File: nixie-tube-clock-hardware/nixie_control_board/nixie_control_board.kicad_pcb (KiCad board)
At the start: 2 copper layers, 52.5 x 97 mm, 62 parts, among them J1 Conn_01x07, P1 CONN_01X02, P2 CONN_01X02, P3 AMS1117, P4 CONN_01X02, P6 CONN_01X02, P7 CONN_01X02, Q1 IRF644, SW4 SW_DIP_x01, U1 DS3231, U2 AT24C02, U3 MAX1771, U7 SSD1306-OLED, U8 MP2307

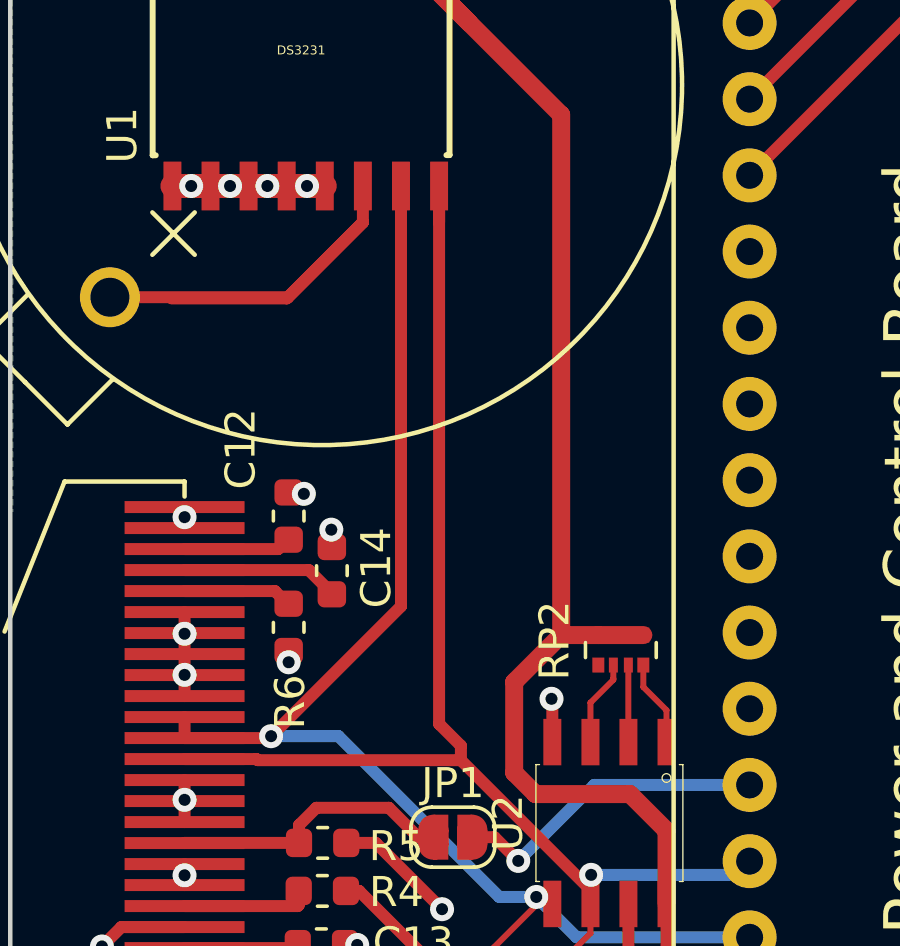
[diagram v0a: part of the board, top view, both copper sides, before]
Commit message: Some hardware changes
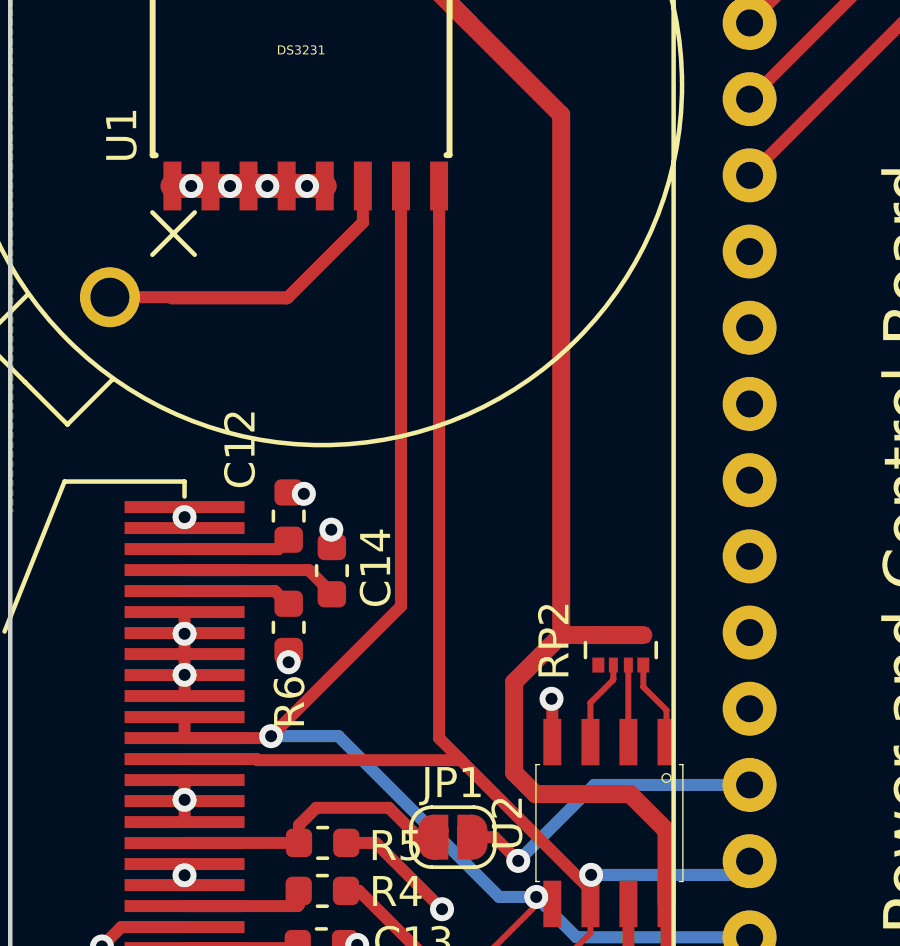
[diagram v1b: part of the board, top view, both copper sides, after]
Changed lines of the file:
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@@
   )
   (setup
-    (last_trace_width 0.4)
+    (last_trace_width 0.2)
     (user_trace_width 0.2)
     (user_trace_width 0.4)
@@
   (segment (start 139.85974 94.15008) (end 139.85974 93.6751) (width 0.4) (layer F.Cu) (net 14))
   (segment (start 134.8142 71.4303) (end 134.8142 70.2178) (width 0.4) (layer F.Cu) (net 14))
-  (segment (start 135.541641 88.875559) (end 134.8142 88.148118) (width 0.4) (layer F.Cu) (net 14))
-  (segment (start 134.8142 88.148118) (end 134.8142 70.2178) (width 0.4) (layer F.Cu) (net 14))
-  (segment (start 135.541641 89.357001) (end 135.541641 88.875559) (width 0.4) (layer F.Cu) (net 14))
+  (segment (start 135.541641 89.357001) (end 135.541641 89.353241) (width 0.4) (layer F.Cu) (net 14))
+  (segment (start 134.8142 88.6258) (end 134.8142 70.2178) (width 0.4) (layer F.Cu) (net 14))
+  (segment (start 135.541641 89.353241) (end 134.8142 88.6258) (width 0.4) (layer F.Cu) (net 14))
   (segment (start 126.33 87.920038) (end 126.33 88.620036) (width 0.4) (layer F.Cu) (net 15))
   (segment (start 136.6434 95.9128) (end 136.6434 96.3628) (width 0.2) (layer F.Cu) (net 15))

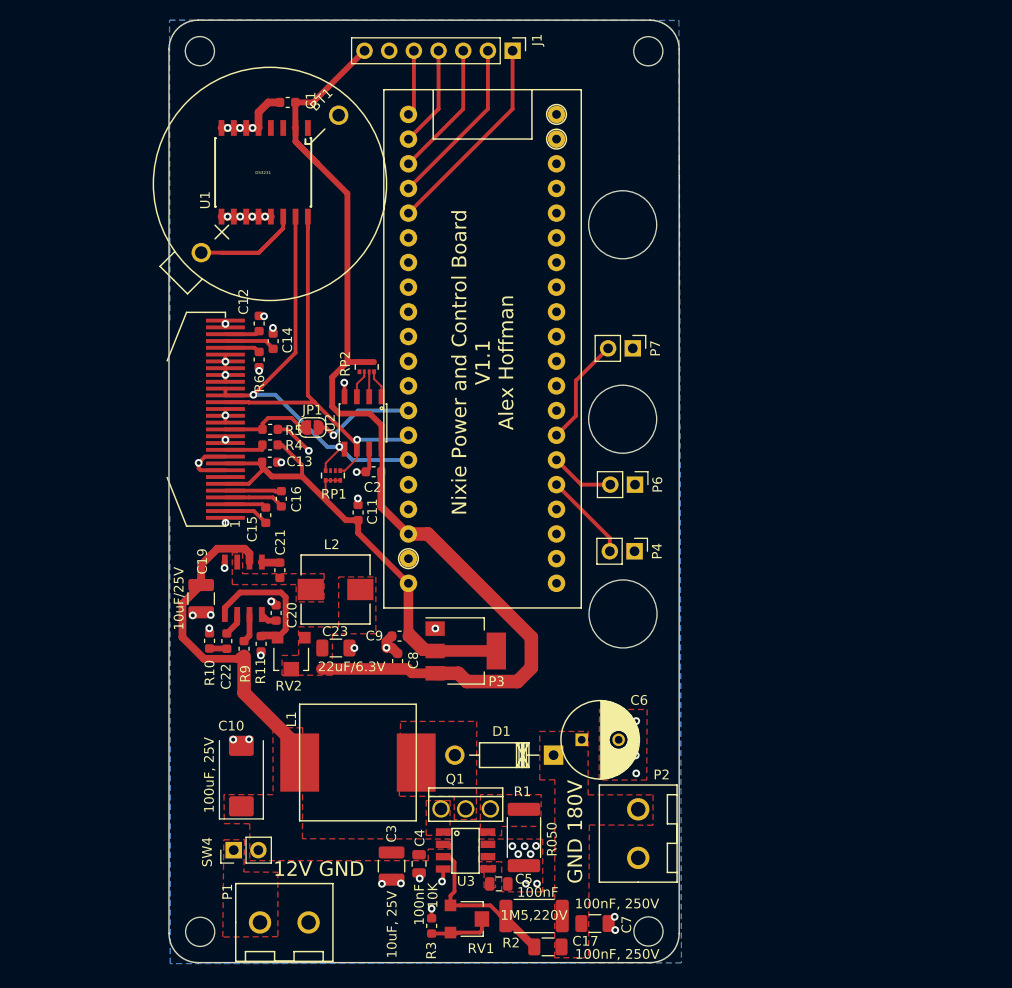
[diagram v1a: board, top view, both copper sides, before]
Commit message: First fixup after looking at this after 2 years
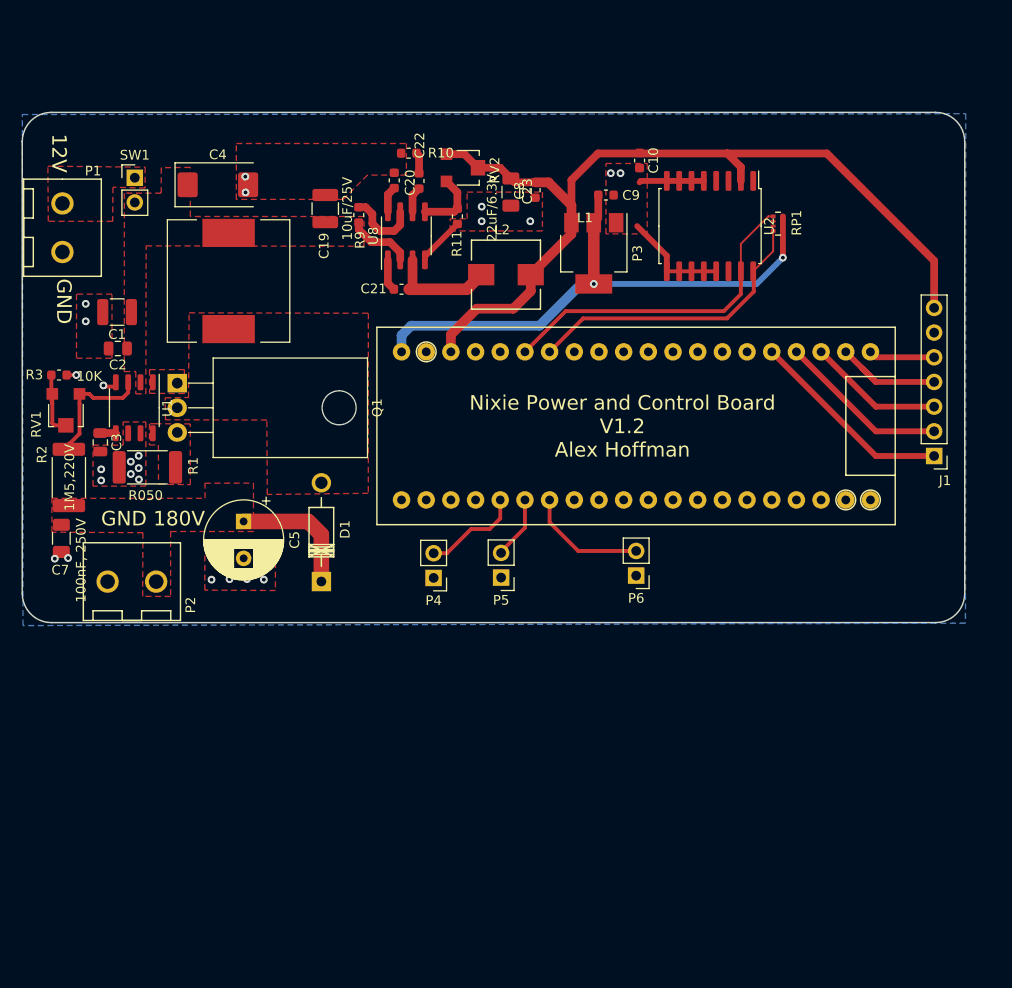
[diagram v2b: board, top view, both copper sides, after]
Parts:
- removed BT1: Battery, keyboard:Coin_battery
- removed C11, C13, C14, C15, C16: 2.2uF, Capacitor_SMD:C_0603_1608Metric
- removed C12: 10uF, Capacitor_SMD:C_0603_1608Metric
- removed C17: 100nF, 250V, Capacitor_SMD:C_1206_3216Metric
- removed C6: 4.7uF/250V, Capacitors_THT:C_Radial_D8_L13_P3.8
- removed JP1: SolderJumper_2_Open, Jumper:SolderJumper-2_P1.3mm_Open_RoundedPad1.0x1.5mm
- removed P7: CONN_01X02, Connector_PinHeader_2.54mm:PinHeader_1x02_P2.54mm_Vertical
- removed R4, R5: 10K, Resistor_SMD:R_0603_1608Metric
- removed R6: 390K, Resistor_SMD:R_0603_1608Metric
- removed REF** (x7): MountingHole_3mm, Mounting_Holes:MountingHole_3mm
- removed RP2: R_PACK4, Resistors_SMD:R_Array_Convex_4x0402
- removed SW4: SW_DIP_x01, Connector_PinHeader_2.54mm:PinHeader_1x02_P2.54mm_Vertical
- removed U3: MAX1771, keyboard_extended:sop-8
- removed U7: SSD1306-OLED, ssd1306oled:SSD1306-096-INCH-OLED
- added P5: CONN_01X02, Connector_PinHeader_2.54mm:PinHeader_1x02_P2.54mm_Vertical, F.Cu at (154.7, 107.4)
- added SW1: SW_DIP_x01, Connector_PinHeader_2.54mm:PinHeader_1x02_P2.54mm_Vertical, F.Cu at (117.0, 66.2)
- C1: value 1uF -> 10uF, 25V; footprint Capacitor_SMD:C_0603_1608Metric -> Capacitor_SMD:C_1210_3225Metric
- C10: value 100uF, 25V -> 1uF; footprint Capacitor_Tantalum_SMD:CP_EIA-7343-15_Kemet-W -> Capacitor_SMD:C_0603_1608Metric
- C2: value 0.1uF -> 100nF; footprint Capacitor_SMD:C_0603_1608Metric -> Capacitor_SMD:C_0805_2012Metric
- C3: value 10uF, 25V -> 100nF; footprint Capacitor_SMD:C_1210_3225Metric -> Capacitor_SMD:C_0805_2012Metric
- C4: value 100nF -> 100uF, 25V; footprint Capacitor_SMD:C_0805_2012Metric -> Capacitor_Tantalum_SMD:CP_EIA-7343-15_Kemet-W
- C5: value 100nF -> 4.7uF/250V; footprint Capacitor_SMD:C_0805_2012Metric -> Capacitor_THT:CP_Radial_D8.0mm_P3.80mm
- L1: footprint keyboard:CD127 -> Inductor_SMD:L_12x12mm_H8mm
- P3: footprint keyboard:SOT-223 -> Package_TO_SOT_SMD:SOT-223
- Q1: footprint keyboard:TO-220 -> Package_TO_SOT_THT:TO-220-3_Horizontal_TabDown
- RP1: value R_PACK4 -> 4K7
- U1: value DS3231 -> MAX1771; footprint keyboard:DS3231 -> Package_SO:SOP-8_3.9x4.9mm_P1.27mm
- U2: value AT24C02 -> DS3231; footprint SMD_Packages:SOIC8 -> Package_SO:SOIC-16W_7.5x10.3mm_P1.27mm
- U8: footprint kicad-libraries:SOIC8 -> Package_SO:SOIC-8_3.9x4.9mm_P1.27mm
- moved C10 75.5 mm to (169.0, 64.4), turned to -90 degrees
- moved P1 75.1 mm to (109.6, 71.4), turned to -90 degrees
- moved C4 72.9 mm to (125.6, 66.9), turned to 0 degrees
- moved R3 68.4 mm to (109.2, 86.5), turned to 0 degrees
- moved C7 67.7 mm to (109.4, 103.3), turned to -90 degrees
- moved RV1 66.7 mm to (109.9, 90.1), turned to 180 degrees
- moved R2 65.8 mm to (110.2, 97.1), turned to 90 degrees
- moved J1 60.2 mm to (199.3, 94.9), turned to 180 degrees
- moved P2 58.2 mm to (116.7, 107.8), turned to 0 degrees
- moved R1 54.3 mm to (118.3, 96.0), turned to 180 degrees
- moved R10 54.2 mm to (145.2, 63.7), turned to 0 degrees
- moved RV2 53.0 mm to (150.7, 65.2), turned to -90 degrees
- moved Q1 52.9 mm to (121.4, 87.4), turned to -90 degrees
- moved C3 52.9 mm to (113.5, 93.4)
- moved RP1 52.6 mm to (183.2, 70.9), turned to 180 degrees
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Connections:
- C1 pad 1: +5V -> +12V
- C10 pad 1: +12V -> +5V
- C2 pad 1: GND -> +12V
- C2 pad 2: +5V -> GND
- C3 pad 1: +12V -> Net-(C3-Pad1)
- C7 pad 1: Net-(C17-Pad1) -> Net-(C5-Pad1)
- D1 pad 1: Net-(C17-Pad1) -> Net-(C5-Pad1)
- MCU1 pad 10: Net-(MCU1-Pad10) -> unconnected-(MCU1-Pad10)
- MCU1 pad 12: Net-(MCU1-Pad12) -> unconnected-(MCU1-Pad12)
- MCU1 pad 13: Net-(MCU1-Pad13) -> unconnected-(MCU1-Pad13)
- MCU1 pad 17: Net-(MCU1-Pad17) -> unconnected-(MCU1-Pad17)
- MCU1 pad 18: Net-(MCU1-Pad18) -> unconnected-(MCU1-Pad18)
- MCU1 pad 19: Net-(MCU1-Pad19) -> unconnected-(MCU1-Pad19)
- MCU1 pad 20: Net-(MCU1-Pad20) -> unconnected-(MCU1-Pad20)
- MCU1 pad 24: Net-(MCU1-Pad24) -> unconnected-(MCU1-Pad24)
- MCU1 pad 25: Net-(MCU1-Pad25) -> unconnected-(MCU1-Pad25)
- MCU1 pad 28: /RESET -> /Controller/RESET
- MCU1 pad 29: Net-(MCU1-Pad29) -> unconnected-(MCU1-Pad29)
- MCU1 pad 3: Net-(MCU1-Pad3) -> unconnected-(MCU1-Pad3)
- MCU1 pad 30: Net-(MCU1-Pad30) -> unconnected-(MCU1-Pad30)
- MCU1 pad 31: Net-(MCU1-Pad31) -> unconnected-(MCU1-Pad31)
- MCU1 pad 32: Net-(MCU1-Pad32) -> unconnected-(MCU1-Pad32)
- MCU1 pad 33: Net-(MCU1-Pad33) -> unconnected-(MCU1-Pad33)
- MCU1 pad 34: Net-(MCU1-Pad34) -> unconnected-(MCU1-Pad34)
- MCU1 pad 35: Net-(MCU1-Pad35) -> unconnected-(MCU1-Pad35)
- MCU1 pad 4: Net-(MCU1-Pad4) -> unconnected-(MCU1-Pad4)
- MCU1 pad 7: Net-(MCU1-Pad7) -> unconnected-(MCU1-Pad7)
- MCU1 pad 8: Net-(MCU1-Pad8) -> unconnected-(MCU1-Pad8)
- P2 pad 2: Net-(C17-Pad1) -> Net-(C5-Pad1)
- P6 pad 2: BUTTON_2 -> BUTTON_3
- Q1 pad 1: Net-(D1-Pad2) -> Net-(U1-Pad1)
- Q1 pad 2: Net-(Q1-Pad2) -> Net-(D1-Pad2)
- Q1 pad 3: Net-(Q1-Pad3) -> Net-(R1-Pad1)
- R1 pad 1: Net-(Q1-Pad3) -> Net-(R1-Pad1)
- R2 pad 1: Net-(C17-Pad1) -> Net-(C5-Pad1)
- R2 pad 2: Net-(C17-Pad2) -> Net-(R2-Pad2)
- RP1 pad 5: SCL -> SDA
- RP1 pad 6: Net-(RP1-Pad6) -> unconnected-(RP1-Pad6)
- RP1 pad 7: Net-(RP1-Pad7) -> unconnected-(RP1-Pad7)
- RP1 pad 8: SDA -> SCL
- RV1 pad 1: Net-(C17-Pad2) -> Net-(R2-Pad2)
- U1 pad 1: Net-(P5-Pad1) -> Net-(U1-Pad1)
- U1 pad 2: +5V -> +12V
- U1 pad 3: SQW -> Net-(R2-Pad2)
- U1 pad 4: Net-(U1-Pad4) -> GND
- U1 pad 5: GND -> Net-(C3-Pad1)
- U1 pad 8: GND -> Net-(R1-Pad1)
- U2 pad 1: Net-(RP2-Pad8) -> unconnected-(U2-Pad1)
- U2 pad 2: Net-(RP2-Pad7) -> +5V
- U2 pad 3: Net-(RP2-Pad6) -> SQW
- U2 pad 4: GND -> unconnected-(U2-Pad4)
- U2 pad 5: SDA -> GND
- U2 pad 6: SCL -> GND
- U2 pad 8: +5V -> GND
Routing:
- net SCL: track 61.5 -> 31.7 mm, vias 1 -> 0
- net +12V: track 34.5 -> 6.72 mm
- net GND: track 47.1 -> 27.0 mm, vias 51 -> 24
- net +5V: track 110.6 -> 91.5 mm
- net Net-(BT1-Pad1): track 18.1 -> 0.00 mm
- net Net-(C17-Pad2): track 16.8 -> 0.00 mm
- net Net-(C5-Pad1): track 0.00 -> 13.4 mm
- net Net-(R2-Pad2): track 0.00 -> 12.7 mm
- net Net-(C21-Pad1): track 0.00 -> 11.2 mm
- net SDA: track 45.8 -> 34.7 mm, vias 2 -> 0
- net /RESET: track 10.6 -> 0.00 mm, vias 1 -> 0
- net Net-(JP1-Pad1): track 9.53 -> 0.00 mm
- net Net-(R11-Pad2): track 15.7 -> 6.75 mm
- net Net-(C16-Pad1): track 6.13 -> 0.00 mm
- net Net-(C16-Pad2): track 5.79 -> 0.00 mm
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- added copper zone on F.Cu, net Net-(R1-Pad1)
- added copper zone on F.Cu, net Net-(U1-Pad1)
- removed copper zone on F.Cu, net +5V
- removed copper zone on F.Cu, net Net-(C17-Pad1)
- removed copper zone on F.Cu, net Net-(C21-Pad1)
- removed copper zone on F.Cu, net Net-(Q1-Pad2)
- removed copper zone on F.Cu, net Net-(Q1-Pad3)
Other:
- board size 52.5 x 97 mm -> 97 x 52.5 mm
- net class Default removed
- board text added: "12V"
- board text added: "GND"
- board text added: "Nixie Power and Control Board V1.2 Alex Hoffman"
- board text removed: "12V GND"
- board text removed: "Nixie Power and Control Board V1.1 Alex Hoffman"

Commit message: V1.2 Control board
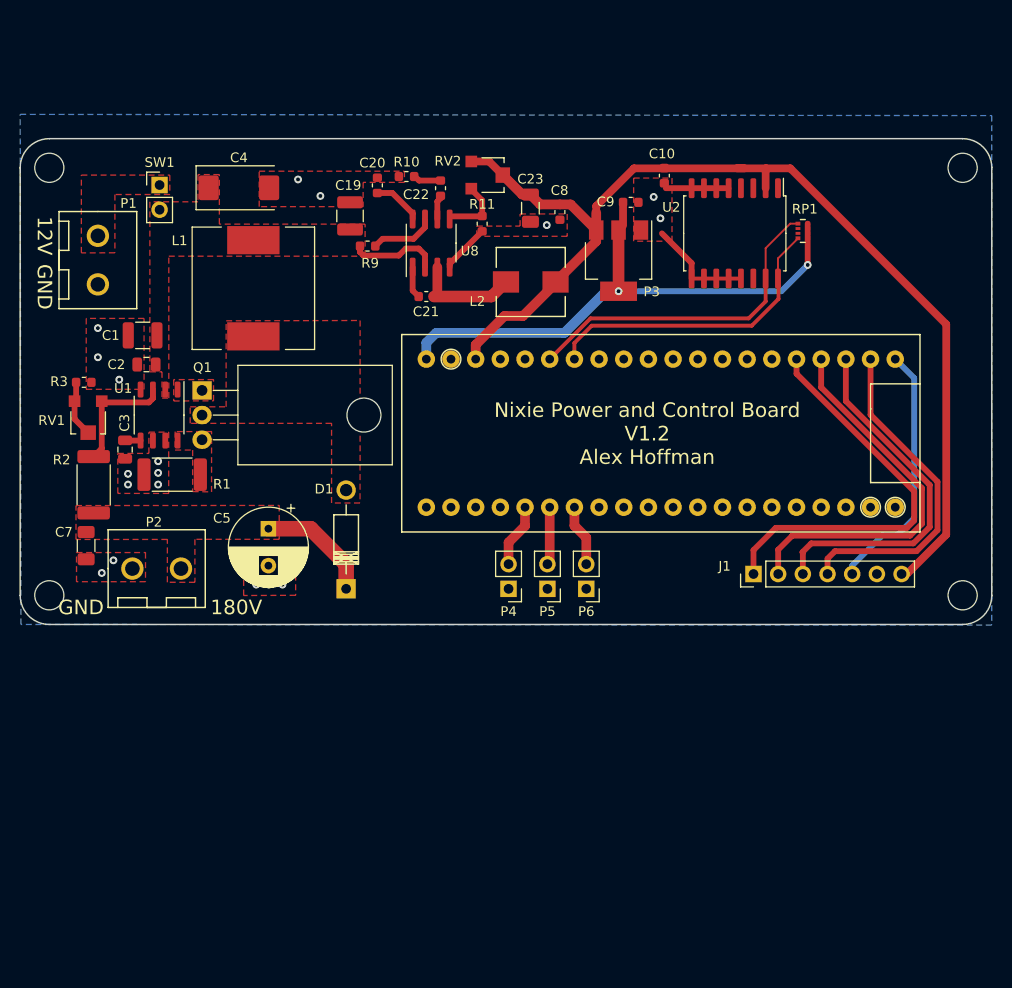
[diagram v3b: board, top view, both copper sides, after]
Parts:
- added REF**: MountingHole_3mm, Mounting_Holes:MountingHole_3mm, F.Cu at (202.2, 109.2)
- added REF**: MountingHole_3mm, Mounting_Holes:MountingHole_3mm, F.Cu at (108.2, 65.2)
- added REF**: MountingHole_3mm, Mounting_Holes:MountingHole_3mm, F.Cu at (202.2, 65.2)
- added REF**: MountingHole_3mm, Mounting_Holes:MountingHole_3mm, F.Cu at (108.2, 109.2)
- moved J1 22.2 mm to (180.7, 107.0), turned to 90 degrees
- moved P4 7.79 mm to (155.5, 108.5)
- moved P6 5.31 mm to (163.5, 108.5)
- moved P1 4.94 mm to (113.2, 74.7)
- moved P5 4.90 mm to (159.5, 108.5)
- moved C1 3.56 mm to (117.8, 82.4)
- moved C8 3.41 mm to (160.8, 69.8)
- moved C2 3.38 mm to (118.2, 85.4)
- moved R9 3.34 mm to (141.0, 73.3), turned to 180 degrees
- moved C10 2.99 mm to (171.5, 66.0)
- moved P2 2.88 mm to (119.3, 106.4)
- moved C19 2.66 mm to (139.2, 70.1)
- moved C21 2.66 mm to (147.0, 78.4)
- moved C5 2.66 mm to (130.8, 102.3)
- moved C9 2.66 mm to (168.0, 68.8)
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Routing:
- net SHIFT_LATCH_CLOCK: track 14.0 -> 37.3 mm
- net SHIFT_SERIAL_CLOCK: track 12.4 -> 34.6 mm
- net SHIFT_OUT_ENABLE: track 17.6 -> 39.6 mm
- net +5V: track 91.5 -> 112.8 mm
- net SHIFT_CLEAR: track 21.2 -> 41.9 mm
- net SHIFT_SER_OUT: track 6.78 -> 26.4 mm
- net BUTTON_3: track 12.4 -> 6.37 mm
- net GND: track 27.0 -> 22.5 mm, vias 24 -> 18
- net BUTTON_1: track 10.2 -> 6.56 mm
- net +12V: track 6.72 -> 9.29 mm
- net Net-(C20-Pad2): track 2.71 -> 5.12 mm
- net Net-(R3-Pad1): track 7.62 -> 5.96 mm
- net Net-(C5-Pad1): track 13.4 -> 12.0 mm
- net SCL: track 31.7 -> 32.7 mm
- net Net-(C22-Pad1): track 2.17 -> 2.96 mm
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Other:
- board size 97 x 52.5 mm -> 100 x 50 mm
- board text added: "180V"
- board text removed: "GND 180V"
